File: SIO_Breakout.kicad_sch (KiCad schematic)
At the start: 2 parts, among them J1 Atari_SIO_Connector, J2 Conn_01x13

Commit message: Layout Complete
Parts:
- J1: footprint (none) -> Atari:Atari_SIO_Socket
- J2: footprint (none) -> Connector_PinHeader_2.54mm:PinHeader_1x13_P2.54mm_Horizontal
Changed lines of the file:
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@@
 			)
 		)
-		(property "Footprint" ""
+		(property "Footprint" "Atari:Atari_SIO_Socket"
 			(at 114.3 109.22 0)
 			(effects
@@
 			)
 		)
-		(property "Footprint" ""
+		(property "Footprint" "Connector_PinHeader_2.54mm:PinHeader_1x13_P2.54mm_Horizontal"
 			(at 189.23 100.33 0)
 			(effects

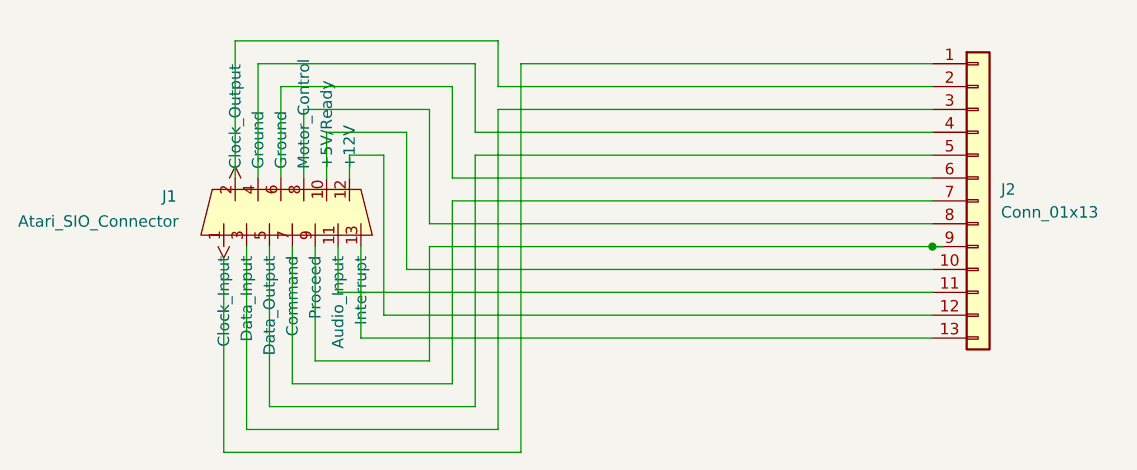
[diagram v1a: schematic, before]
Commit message: Rules Checking
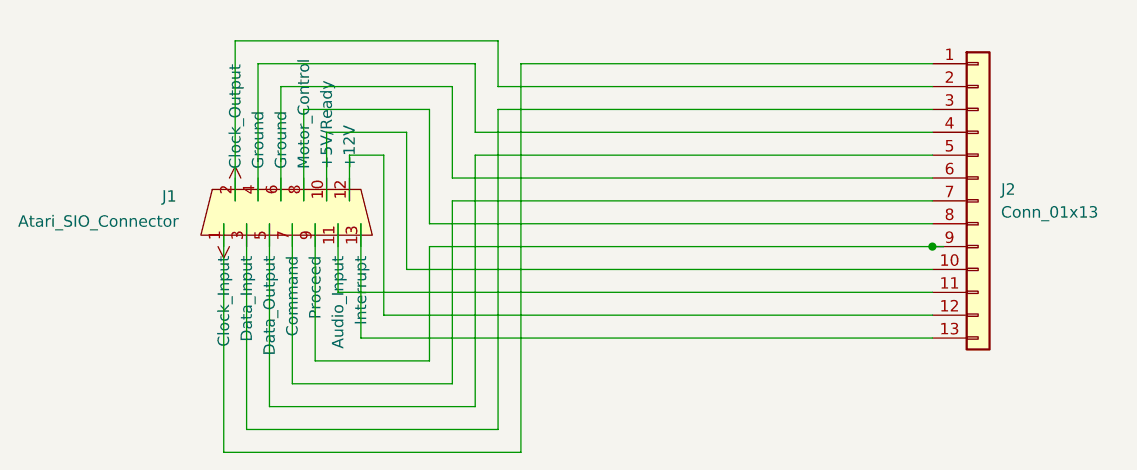
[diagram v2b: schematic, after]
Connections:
- net at J1.1 (Clock_Input): now also J2.1 (Pin_1)
- net at J1.10 (+5V/Ready): now also J2.10 (Pin_10)
- net at J1.11 (Audio_Input): now also J2.11 (Pin_11)
- net at J1.12 (+12V): now also J2.12 (Pin_12)
- net at J1.13 (Interrupt): now also J2.13 (Pin_13)
- net at J1.2 (Clock_Output): now also J2.2 (Pin_2)
- net at J1.3 (Data_Input): now also J2.3 (Pin_3)
- net at J1.4 (Ground): now also J2.4 (Pin_4)
- net at J1.5 (Data_Output): now also J2.5 (Pin_5)
- net at J1.6 (Ground): now also J2.6 (Pin_6)
- net at J1.7 (Command): now also J2.7 (Pin_7)
- net at J1.8 (Motor_Control): now also J2.8 (Pin_8)
- net at J1.9 (Proceed): now also J2.9 (Pin_9)
